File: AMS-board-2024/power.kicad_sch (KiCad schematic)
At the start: 64 parts, among them Q109 DMT6007LFGQ, Q110 BSS308PE, Q111 2N7002K-AU, Q112 2N7002K-AU, Q113 DMT6007LFGQ, Q114 2N7002K-AU, U18 UCC12040, U19 AP74700QW6-7, U20 VOMA617A, U21 LM5060, U22 LMR33630APCQRNXRQ1

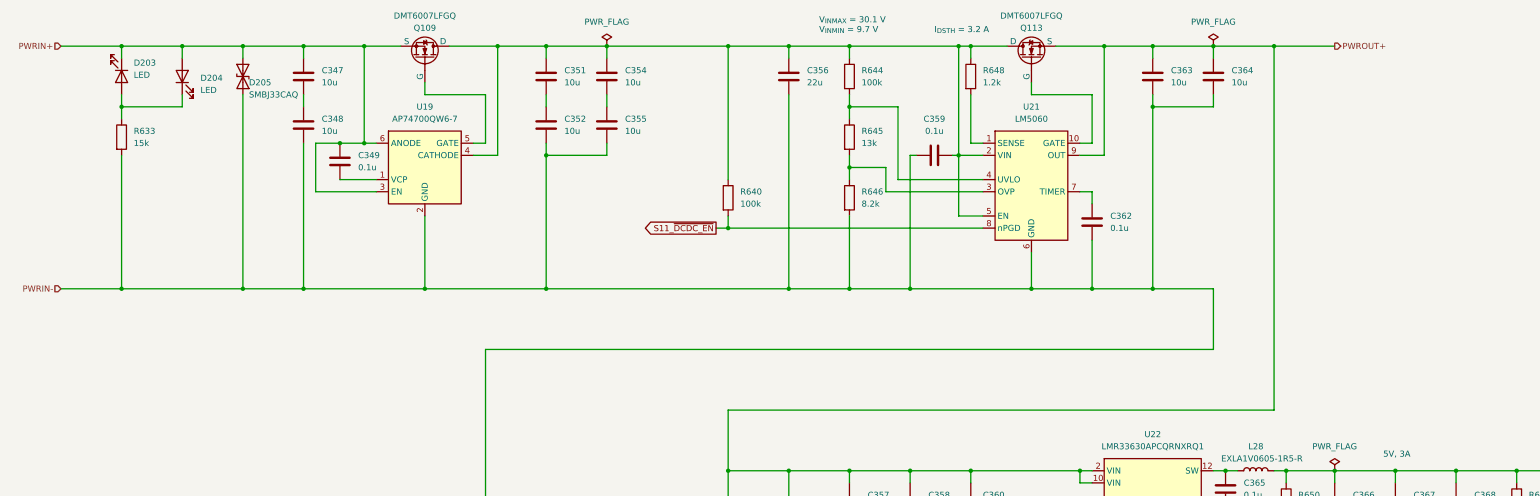
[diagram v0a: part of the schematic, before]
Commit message: ヒューズ追加
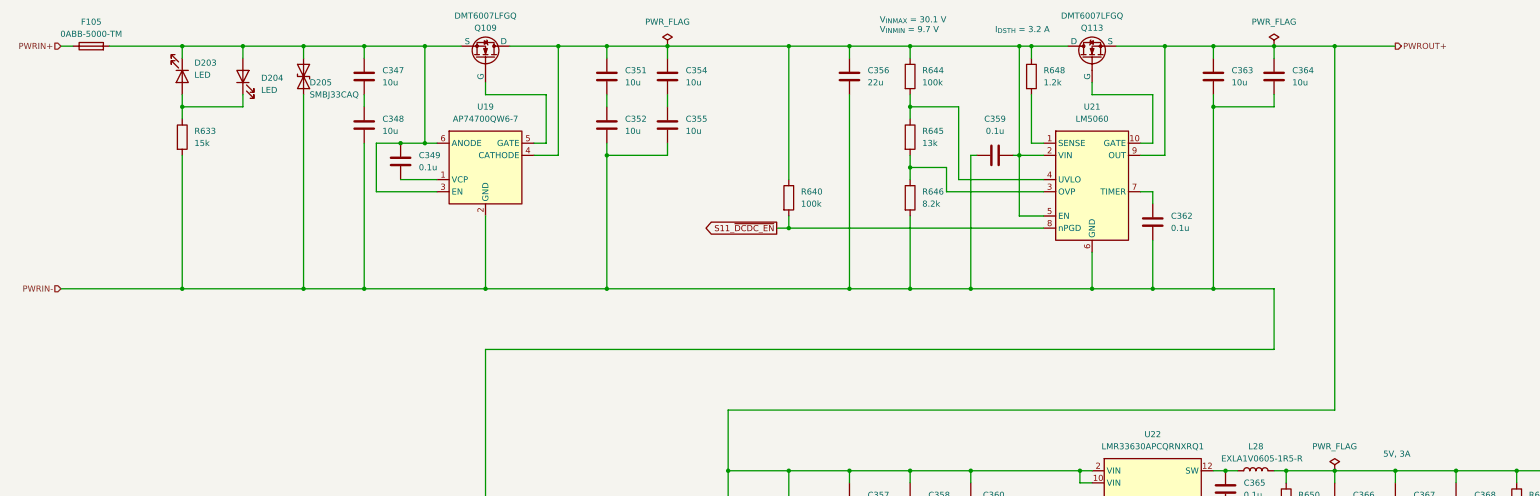
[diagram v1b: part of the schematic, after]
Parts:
- added F105: 0ABB-5000-TM, ProjectEV:Fuse_0ABB, symbol ProjectEV:Fuse_0ABB-5000-TM
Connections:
- net PWRIN+: now also F105.1; no longer C347.1, C349.1, D203.1 (K), D204.2 (A), D205.2 (A2), Q109.1 (S), Q109.2 (S), Q109.3 (S), U19.3 (EN), U19.6 (ANODE)
- new net: C347.1, C349.1, D203.1 (K), D204.2 (A), D205.2 (A2), F105.2, Q109.1 (S), Q109.2 (S), Q109.3 (S), U19.3 (EN), U19.6 (ANODE)
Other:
- moved on the sheet: C347, C348, C349, C351, C352, C354, C355, C356, C359, C362, C363, C364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

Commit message: チップ抵抗、チップコンデンササイズ修正
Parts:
- C346, C349, C350, C359, C360, C361, C362, C365, C366: footprint Capacitor_SMD:C_0603_1608Metric -> Capacitor_SMD:C_0402_1005Metric
- C367, C368: footprint Capacitor_SMD:C_0805_2012Metric -> Capacitor_SMD:C_1206_3216Metric
- R634, R636, R637, R638, R639, R640, R641, R643, R644, R645, R646, R647, R648, R649, R650, R651, R652, R653: footprint Resistor_SMD:R_0603_1608Metric -> Resistor_SMD:R_0402_1005Metric
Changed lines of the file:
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@@
       (effects (font (size 1.27 1.27)) (justify left))
     )
-    (property "Footprint" "Resistor_SMD:R_0603_1608Metric" (at 292.862 146.05 90)
+    (property "Footprint" "Resistor_SMD:R_0402_1005Metric" (at 292.862 146.05 90)
       (effects (font (size 1.27 1.27)) hide)
     )
@@
       (effects (font (size 1.27 1.27)) (justify right))
     )
-    (property "Footprint" "Resistor_SMD:R_0603_1608Metric" (at 173.228 228.6 90)
+    (property "Footprint" "Resistor_SMD:R_0402_1005Metric" (at 173.228 228.6 90)
       (effects (font (size 1.27 1.27)) hide)
     )
@@
       (effects (font (size 1.27 1.27)) (justify left))
     )
-    (property "Footprint" "Resistor_SMD:R_0603_1608Metric" (at 239.522 44.45 90)
+    (property "Footprint" "Resistor_SMD:R_0402_1005Metric" (at 239.522 44.45 90)
       (effects (font (size 1.27 1.27)) hide)
     )
@@
       (effects (font (size 1.27 1.27)) (justify left))
     )
-    (property "Footprint" "Capacitor_SMD:C_0603_1608Metric" (at 267.6652 78.74 0)
+    (property "Footprint" "Capacitor_SMD:C_0402_1005Metric" (at 267.6652 78.74 0)
       (effects (font (size 1.27 1.27)) hide)
     )
@@
       (effects (font (size 1.27 1.27)) (justify left))
     )
-    (property "Footprint" "Capacitor_SMD:C_0805_2012Metric" (at 318.4652 137.16 0)
+    (property "Footprint" "Capacitor_SMD:C_1206_3216Metric" (at 318.4652 137.16 0)
       (effects (font (size 1.27 1.27)) hide)
     )
@@
       (effects (font (size 1.27 1.27)) (justify left))
     )
-    (property "Footprint" "Resistor_SMD:R_0603_1608Metric" (at 201.422 171.45 90)
+    (property "Footprint" "Resistor_SMD:R_0402_1005Metric" (at 201.422 171.45 90)
       (effects (font (size 1.27 1.27)) hide)
     )
@@
       (effects (font (size 1.27 1.27)) (justify left))
     )
-    (property "Footprint" "Capacitor_SMD:C_0805_2012Metric" (at 331.1652 137.16 0)
+    (property "Footprint" "Capacitor_SMD:C_1206_3216Metric" (at 331.1652 137.16 0)
       (effects (font (size 1.27 1.27)) hide)
     )
@@
       (effects (font (size 1.27 1.27)) (justify left))
     )
-    (property "Footprint" "Resistor_SMD:R_0603_1608Metric" (at 188.722 69.85 90)
+    (property "Footprint" "Resistor_SMD:R_0402_1005Metric" (at 188.722 69.85 90)
       (effects (font (size 1.27 1.27)) hide)
     )
@@
       (effects (font (size 1.27 1.27)) (justify left))
     )
-    (property "Footprint" "Resistor_SMD:R_0603_1608Metric" (at 176.022 146.05 90)
+    (property "Footprint" "Resistor_SMD:R_0402_1005Metric" (at 176.022 146.05 90)
       (effects (font (size 1.27 1.27)) hide)
     )
@@
       (effects (font (size 1.27 1.27)))
     )
-    (property "Footprint" "Resistor_SMD:R_0603_1608Metric" (at 328.93 160.528 90)
+    (property "Footprint" "Resistor_SMD:R_0402_1005Metric" (at 328.93 160.528 90)
       (effects (font (size 1.27 1.27)) hide)
     )
@@
       (effects (font (size 1.27 1.27)) (justify left))
     )
-    (property "Footprint" "Resistor_SMD:R_0603_1608Metric" (at 214.122 57.15 90)
+    (property "Footprint" "Resistor_SMD:R_0402_1005Metric" (at 214.122 57.15 90)
       (effects (font (size 1.27 1.27)) hide)
     )
@@
       (effects (font (size 1.27 1.27)))
     )
-    (property "Footprint" "Resistor_SMD:R_0603_1608Metric" (at 171.45 249.428 90)
+    (property "Footprint" "Resistor_SMD:R_0402_1005Metric" (at 171.45 249.428 90)
       (effects (font (size 1.27 1.27)) hide)
     )
@@
       (effects (font (size 1.27 1.27)) (justify left))
     )
-    (property "Footprint" "Capacitor_SMD:C_0603_1608Metric" (at 305.7652 137.16 0)
+    (property "Footprint" "Capacitor_SMD:C_0402_1005Metric" (at 305.7652 137.16 0)
       (effects (font (size 1.27 1.27)) hide)
     )
@@
       (effects (font (size 1.27 1.27)) (justify right))
     )
-    (property "Footprint" "Capacitor_SMD:C_0603_1608Metric" (at 62.5348 218.44 0)
+    (property "Footprint" "Capacitor_SMD:C_0402_1005Metric" (at 62.5348 218.44 0)
       (effects (font (size 1.27 1.27)) hide)
     )
@@
       (effects (font (size 1.27 1.27)) (justify left))
     )
-    (property "Footprint" "Capacitor_SMD:C_0603_1608Metric" (at 110.1852 66.04 0)
+    (property "Footprint" "Capacitor_SMD:C_0402_1005Metric" (at 110.1852 66.04 0)
       (effects (font (size 1.27 1.27)) hide)
     )
@@
       (effects (font (size 1.27 1.27)))
     )
-    (property "Footprint" "Resistor_SMD:R_0603_1608Metric" (at 158.75 160.528 90)
+    (property "Footprint" "Resistor_SMD:R_0402_1005Metric" (at 158.75 160.528 90)
       (effects (font (size 1.27 1.27)) hide)
     )
@@
       (effects (font (size 1.27 1.27)) (justify left))
     )
-    (property "Footprint" "Capacitor_SMD:C_0603_1608Metric" (at 282.9052 134.62 0)
+    (property "Footprint" "Capacitor_SMD:C_0402_1005Metric" (at 282.9052 134.62 0)
       (effects (font (size 1.27 1.27)) hide)
     )
@@
       (effects (font (size 1.27 1.27)) (justify left))
     )
-    (property "Footprint" "Resistor_SMD:R_0603_1608Metric" (at 188.722 222.25 90)
+    (property "Footprint" "Resistor_SMD:R_0402_1005Metric" (at 188.722 222.25 90)
       (effects (font (size 1.27 1.27)) hide)
     )
@@
       (effects (font (size 1.27 1.27)) (justify left))
     )
-    (property "Footprint" "Resistor_SMD:R_0603_1608Metric" (at 150.622 222.25 90)
+    (property "Footprint" "Resistor_SMD:R_0402_1005Metric" (at 150.622 222.25 90)
       (effects (font (size 1.27 1.27)) hide)
     )
@@
       (effects (font (size 1.27 1.27)) (justify left))
     )
-    (property "Footprint" "Resistor_SMD:R_0603_1608Metric" (at 292.862 133.35 90)
+    (property "Footprint" "Resistor_SMD:R_0402_1005Metric" (at 292.862 133.35 90)
       (effects (font (size 1.27 1.27)) hide)
     )
@@
       (effects (font (size 1.27 1.27)) (justify right))
     )
-    (property "Footprint" "Capacitor_SMD:C_0603_1608Metric" (at 126.0348 218.44 0)
+    (property "Footprint" "Capacitor_SMD:C_0402_1005Metric" (at 126.0348 218.44 0)
       (effects (font (size 1.27 1.27)) hide)
     )
@@
       (effects (font (size 1.27 1.27)) (justify left))
     )
-    (property "Footprint" "Resistor_SMD:R_0603_1608Metric" (at 214.122 69.85 90)
+    (property "Footprint" "Resistor_SMD:R_0402_1005Metric" (at 214.122 69.85 90)
       (effects (font (size 1.27 1.27)) hide)
     )
@@
       (effects (font (size 1.27 1.27)) (justify left))
     )
-    (property "Footprint" "Capacitor_SMD:C_0603_1608Metric" (at 229.5652 137.16 0)
+    (property "Footprint" "Capacitor_SMD:C_0402_1005Metric" (at 229.5652 137.16 0)
       (effects (font (size 1.27 1.27)) hide)
     )
@@
       (effects (font (size 1.27 1.27)) (justify left))
     )
-    (property "Footprint" "Resistor_SMD:R_0603_1608Metric" (at 341.122 133.35 90)
+    (property "Footprint" "Resistor_SMD:R_0402_1005Metric" (at 341.122 133.35 90)
       (effects (font (size 1.27 1.27)) hide)
     )
@@
       (effects (font (size 1.27 1.27)) (justify left))
     )
-    (property "Footprint" "Capacitor_SMD:C_0603_1608Metric" (at 252.4252 149.86 0)
+    (property "Footprint" "Capacitor_SMD:C_0402_1005Metric" (at 252.4252 149.86 0)
       (effects (font (size 1.27 1.27)) hide)
     )
@@
       (effects (font (size 1.27 1.27)))
     )
-    (property "Footprint" "Capacitor_SMD:C_0603_1608Metric" (at 237.49 59.9948 0)
+    (property "Footprint" "Capacitor_SMD:C_0402_1005Metric" (at 237.49 59.9948 0)
       (effects (font (size 1.27 1.27)) hide)
     )
@@
       (effects (font (size 1.27 1.27)) (justify left))
     )
-    (property "Footprint" "Resistor_SMD:R_0603_1608Metric" (at 74.422 222.25 90)
+    (property "Footprint" "Resistor_SMD:R_0402_1005Metric" (at 74.422 222.25 90)
       (effects (font (size 1.27 1.27)) hide)
     )
@@
       (effects (font (size 1.27 1.27)))
     )
-    (property "Footprint" "Resistor_SMD:R_0603_1608Metric" (at 246.38 141.478 90)
+    (property "Footprint" "Resistor_SMD:R_0402_1005Metric" (at 246.38 141.478 90)
       (effects (font (size 1.27 1.27)) hide)
     )
@@
       (effects (font (size 1.27 1.27)) (justify left))
     )
-    (property "Footprint" "Resistor_SMD:R_0603_1608Metric" (at 214.122 44.45 90)
-      (effects (font (size 1.27 1.27)) hide)
-    )
+    (property "Footprint" "Resistor_SMD:R_0402_1005Metric" (at 214.122 44.45 90)
+      (effects (font (size 1.27 1.27)) hide)
+    )
